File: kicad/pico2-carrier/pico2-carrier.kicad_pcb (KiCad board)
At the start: 2 copper layers, 1 part, among them U1 Pico 2

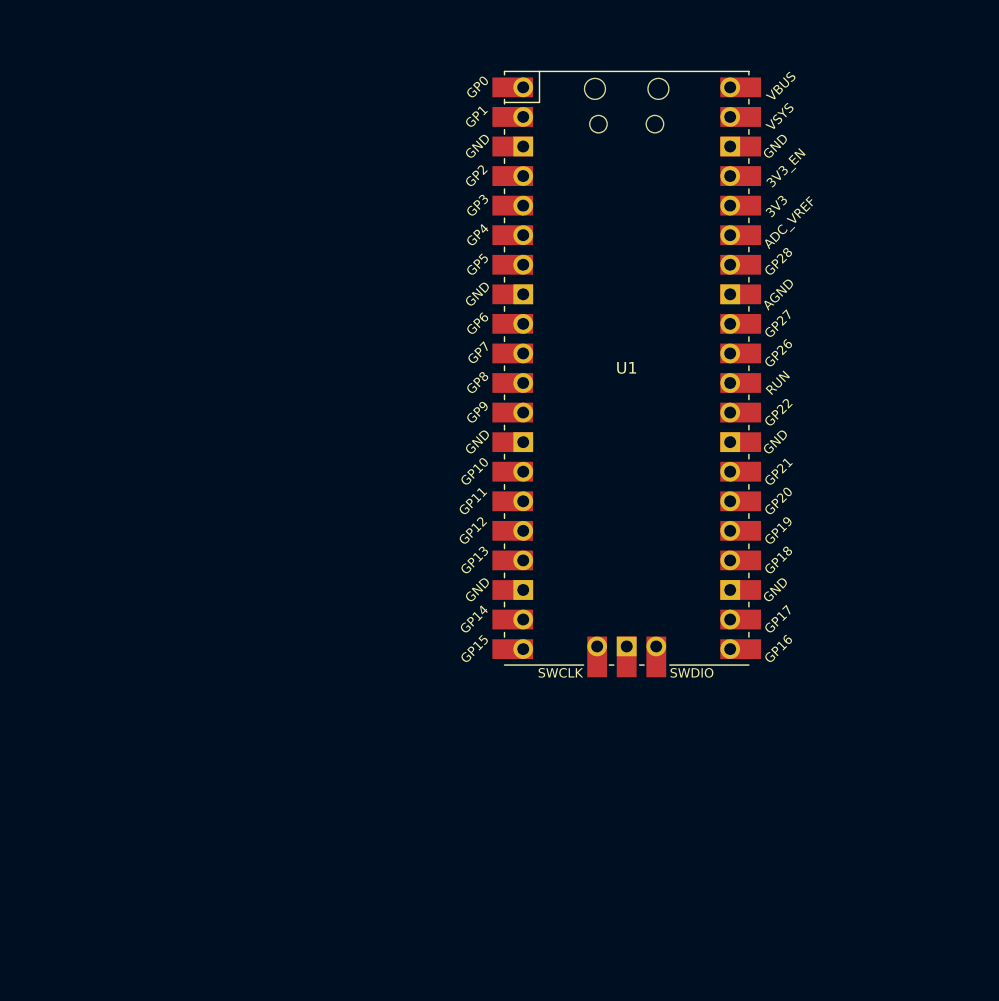
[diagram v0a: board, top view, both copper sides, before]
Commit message: hw: lots of changes to pico 2 board
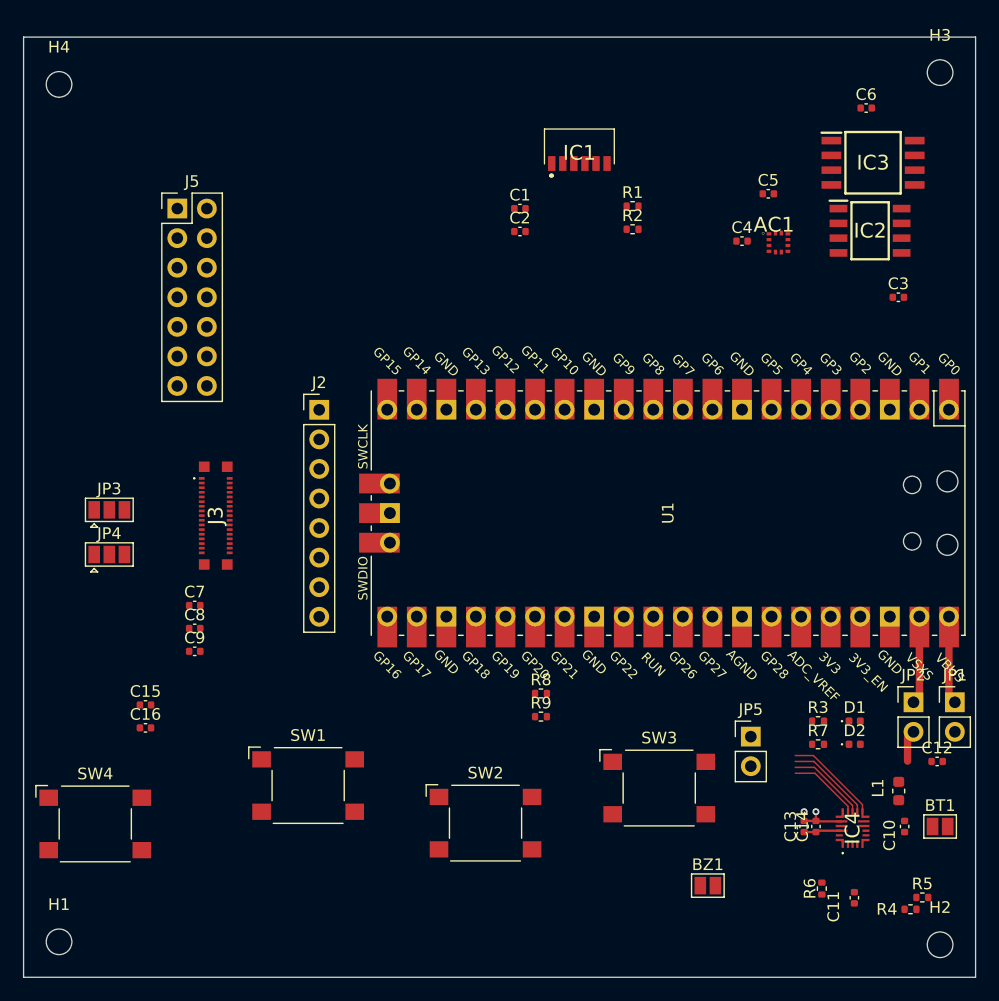
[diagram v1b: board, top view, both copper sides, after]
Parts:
- added AC1: BMA400, SamacsysParts:BOSCH_LGA-12, F.Cu at (162.1, 78.1)
- added BT1: Battery_Cell, Jumper:SolderJumper-2_P1.3mm_Open_Pad1.0x1.5mm, F.Cu at (176.0, 128.3)
- added BZ1: Speaker, Jumper:SolderJumper-2_P1.3mm_Open_Pad1.0x1.5mm, F.Cu at (156.1, 133.3)
- added C1: 0.1uF, Capacitor_SMD:C_0402_1005Metric, F.Cu at (139.9, 75.2)
- added C10: 47nF, Capacitor_SMD:C_0402_1005Metric, F.Cu at (173.0, 128.3)
- added C11: 4.7uF, Capacitor_SMD:C_0402_1005Metric, F.Cu at (168.7, 134.4)
- added C12: 1uF, Capacitor_SMD:C_0402_1005Metric, F.Cu at (175.8, 122.7)
- added C13: 10uF, Capacitor_SMD:C_0402_1005Metric, F.Cu at (164.3, 128.3)
- added C14: 0.1uF, Capacitor_SMD:C_0402_1005Metric, F.Cu at (165.4, 128.3)
- added C15: 20uF, Capacitor_SMD:C_0402_1005Metric, F.Cu at (107.8, 117.8)
- added C16: 10uF, Capacitor_SMD:C_0402_1005Metric, F.Cu at (107.8, 119.8)
- added C2: 4.7uF, Capacitor_SMD:C_0402_1005Metric, F.Cu at (139.9, 77.2)
- added C3: 0.1uF, Capacitor_SMD:C_0402_1005Metric, F.Cu at (172.4, 82.8)
- added C4: 0.1uF, Capacitor_SMD:C_0402_1005Metric, F.Cu at (159.0, 78.0)
- added C5: 0.1uF, Capacitor_SMD:C_0402_1005Metric, F.Cu at (161.3, 73.9)
- added C6: 0.1uF, Capacitor_SMD:C_0402_1005Metric, F.Cu at (169.7, 66.5)
- added C7: 10uF, Capacitor_SMD:C_0402_1005Metric, F.Cu at (112.0, 109.3)
- added C8: 10uF, Capacitor_SMD:C_0402_1005Metric, F.Cu at (112.0, 111.3)
- added C9: 10uF, Capacitor_SMD:C_0402_1005Metric, F.Cu at (112.0, 113.2)
- added D1: PG, LED_SMD:LED_0402_1005Metric, F.Cu at (168.7, 119.2)
- added D2: STAT, LED_SMD:LED_0402_1005Metric, F.Cu at (168.7, 121.2)
- added H1: MountingHole, MountingHole:MountingHole_2.2mm_M2, F.Cu at (100.3, 138.2)
- added H2: MountingHole, MountingHole:MountingHole_2.2mm_M2, F.Cu at (176.0, 138.4)
- added H3: MountingHole, MountingHole:MountingHole_2.2mm_M2, F.Cu at (176.0, 63.5)
- added H4: MountingHole, MountingHole:MountingHole_2.2mm_M2, F.Cu at (100.3, 64.5)
- added IC1: TFBS4711-TT1, SamacsysParts:TFBS4711TT1, F.Cu at (145.0, 69.8)
- added IC2: M95512-DRMN8TP_K, SamacsysParts:SOIC127P600X175-8N, F.Cu at (170.0, 77.1)
- added IC3: IS25WP128F-JBLE, SamacsysParts:SOIC127P790X216-8N, F.Cu at (170.3, 71.2)
- added IC4: BQ25628ERYKR, SamacsysParts:BQ25628ERYKR, F.Cu at (168.5, 128.4)
- added J2: SCREEN_HDR, Connector_PinHeader_2.54mm:PinHeader_1x08_P2.54mm_Vertical, F.Cu at (122.7, 92.5)
- added J3: DO0180FMST08, SamacsysParts:AXE534127, F.Cu at (113.8, 101.6)
- added J5: Ext_Pwr_Rail, Connector_PinHeader_2.54mm:PinHeader_2x07_P2.54mm_Vertical, F.Cu at (110.5, 75.2)
- added JP1: Jumper_2_Open, Connector_PinHeader_2.54mm:PinHeader_1x02_P2.54mm_Vertical, F.Cu at (177.3, 117.6)
- added JP2: Jumper_2_Open, Connector_PinHeader_2.54mm:PinHeader_1x02_P2.54mm_Vertical, F.Cu at (173.7, 117.6)
- added JP3: JP_IM0, Jumper:SolderJumper-3_P1.3mm_Open_Pad1.0x1.5mm, F.Cu at (104.6, 101.1)
- added JP4: JP_IM1, Jumper:SolderJumper-3_P1.3mm_Open_Pad1.0x1.5mm, F.Cu at (104.6, 104.9)
- added JP5: 3V3_CURRENT_SENSE, Connector_PinHeader_2.54mm:PinHeader_1x02_P2.54mm_Vertical, F.Cu at (159.8, 120.5)
- added L1: 1uH, Inductor_SMD:L_0603_1608Metric, F.Cu at (172.5, 125.2)
- added R1: 56R, Resistor_SMD:R_0402_1005Metric, F.Cu at (149.6, 75.0)
- added R2: 47R, Resistor_SMD:R_0402_1005Metric, F.Cu at (149.6, 77.0)
- added R3: 470R, Resistor_SMD:R_0402_1005Metric, F.Cu at (165.5, 119.2)
- added R4: R, Resistor_SMD:R_0402_1005Metric, F.Cu at (173.5, 135.4)
- added R5: R, Resistor_SMD:R_0402_1005Metric, F.Cu at (174.5, 134.4)
- added R6: R, Resistor_SMD:R_0402_1005Metric, F.Cu at (165.9, 133.6)
- added R7: 470R, Resistor_SMD:R_0402_1005Metric, F.Cu at (165.5, 121.2)
- added R8: 10k, Resistor_SMD:R_0402_1005Metric, F.Cu at (141.7, 116.8)
- added R9: 10k, Resistor_SMD:R_0402_1005Metric, F.Cu at (141.7, 118.8)
- added SW1: BUT_L, Button_Switch_SMD:SW_SPST_Omron_B3FS-101xP, F.Cu at (121.7, 124.8)
- added SW2: BUT_M, Button_Switch_SMD:SW_SPST_Omron_B3FS-101xP, F.Cu at (137.0, 128.0)
- added SW3: BUT_R, Button_Switch_SMD:SW_SPST_Omron_B3FS-101xP, F.Cu at (151.9, 125.0)
- added SW4: RUN, Button_Switch_SMD:SW_SPST_Omron_B3FS-101xP, F.Cu at (103.4, 128.1)
- moved U1 12.9 mm to (152.7, 101.3), turned to -90 degrees
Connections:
- U1 pad 1: unconnected-(U1-GPIO0-Pad1) -> /DBG_TX
- U1 pad 10: unconnected-(U1-GPIO7-Pad10) -> /ACCEL_INT1
- U1 pad 11: unconnected-(U1-GPIO8-Pad11) -> /~{FLASH_CSB}
- U1 pad 12: unconnected-(U1-GPIO9-Pad12) -> /IR_SD
- U1 pad 13: unconnected-(U1-GND-Pad13) -> GND
- U1 pad 14: unconnected-(U1-GPIO10-Pad14) -> /IR_PIO_RX
- U1 pad 15: unconnected-(U1-GPIO11-Pad15) -> /IR_PIO_TX
- U1 pad 16: unconnected-(U1-GPIO12-Pad16) -> /~{SCREEN_RST}
- U1 pad 17: unconnected-(U1-GPIO13-Pad17) -> /HSTX_SD0
- U1 pad 18: unconnected-(U1-GND-Pad18) -> GND
- U1 pad 19: unconnected-(U1-GPIO14-Pad19) -> /HSTX_SD1
- U1 pad 2: unconnected-(U1-GPIO1-Pad2) -> /DBG_RX
- U1 pad 20: unconnected-(U1-GPIO15-Pad20) -> /HSTX_SCK
- U1 pad 21: unconnected-(U1-GPIO16-Pad21) -> /HSTX_SD2
- U1 pad 22: unconnected-(U1-GPIO17-Pad22) -> /HSTX_SD3
- U1 pad 23: unconnected-(U1-GND-Pad23) -> GND
- U1 pad 24: unconnected-(U1-GPIO18-Pad24) -> /~{SCREEN_CSB}
- U1 pad 25: unconnected-(U1-GPIO19-Pad25) -> /~{BAT_INT}
- U1 pad 26: unconnected-(U1-GPIO20-Pad26) -> /I2C_SDA
- U1 pad 27: unconnected-(U1-GPIO21-Pad27) -> /I2C_SCL
- U1 pad 28: unconnected-(U1-GND-Pad28) -> GND
- U1 pad 29: unconnected-(U1-GPIO22-Pad29) -> /BUT_L
- U1 pad 3: unconnected-(U1-GND-Pad3) -> GND
- U1 pad 30: unconnected-(U1-RUN-Pad30) -> /RUN
- U1 pad 31: unconnected-(U1-GPIO26_ADC0-Pad31) -> /BUT_M
- U1 pad 32: unconnected-(U1-GPIO27_ADC1-Pad32) -> /BUT_R
- U1 pad 33: unconnected-(U1-AGND-Pad33) -> GND
- U1 pad 34: unconnected-(U1-GPIO28_ADC2-Pad34) -> GND
- U1 pad 35: unconnected-(U1-ADC_VREF-Pad35) -> Net-(JP5-A)
- U1 pad 36: unconnected-(U1-3V3-Pad36) -> Net-(JP5-A)
- U1 pad 38: unconnected-(U1-GND-Pad38) -> GND
- U1 pad 39: unconnected-(U1-VSYS-Pad39) -> Net-(JP2-A)
- U1 pad 4: unconnected-(U1-GPIO2-Pad4) -> /SPI_SCK
- U1 pad 40: unconnected-(U1-VBUS-Pad40) -> Net-(JP1-A)
- U1 pad 41: unconnected-(U1-SWCLK-Pad41) -> /SWCLK
- U1 pad 42: unconnected-(U1-GND-Pad42) -> GND
- U1 pad 43: unconnected-(U1-SWDIO-Pad43) -> /SWDIO
- U1 pad 5: unconnected-(U1-GPIO3-Pad5) -> /SPI_MOSI
- U1 pad 6: unconnected-(U1-GPIO4-Pad6) -> /SPI_MISO
- U1 pad 7: unconnected-(U1-GPIO5-Pad7) -> /~{EEPROM_CSB}
- U1 pad 8: unconnected-(U1-GND-Pad8) -> GND
- U1 pad 9: unconnected-(U1-GPIO6-Pad9) -> /~{ACCEL_CSB}
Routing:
- net Net-(JP1-A): track 0.00 -> 8.29 mm
- net /battery-bq25628e/STAT: track 0.00 -> 8.25 mm
- net Net-(JP2-A): track 0.00 -> 7.57 mm
- net /~{BAT_INT}: track 0.00 -> 7.47 mm
- net /I2C_SDA: track 0.00 -> 6.82 mm
- net /I2C_SCL: track 0.00 -> 6.18 mm
- net GND: track 0.00 -> 4.81 mm, vias 0 -> 2
- net /battery-bq25628e/PMID: track 0.00 -> 3.26 mm
- net VSYS: track 0.00 -> 2.73 mm
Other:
- board outline added: 81.8 x 80.8 mm
- board text added: "AMOLED screen size"
